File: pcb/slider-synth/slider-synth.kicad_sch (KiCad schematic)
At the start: 21 parts, among them J1 USB4105, J2 PJ-325C5-G, J3 Conn_01x02_Pin, SW1 SW_SPST, SW2 SW_SPST, U1 ESP32-S3-WROOM-2, U2 LM3940IMPX-3.3/NOPB

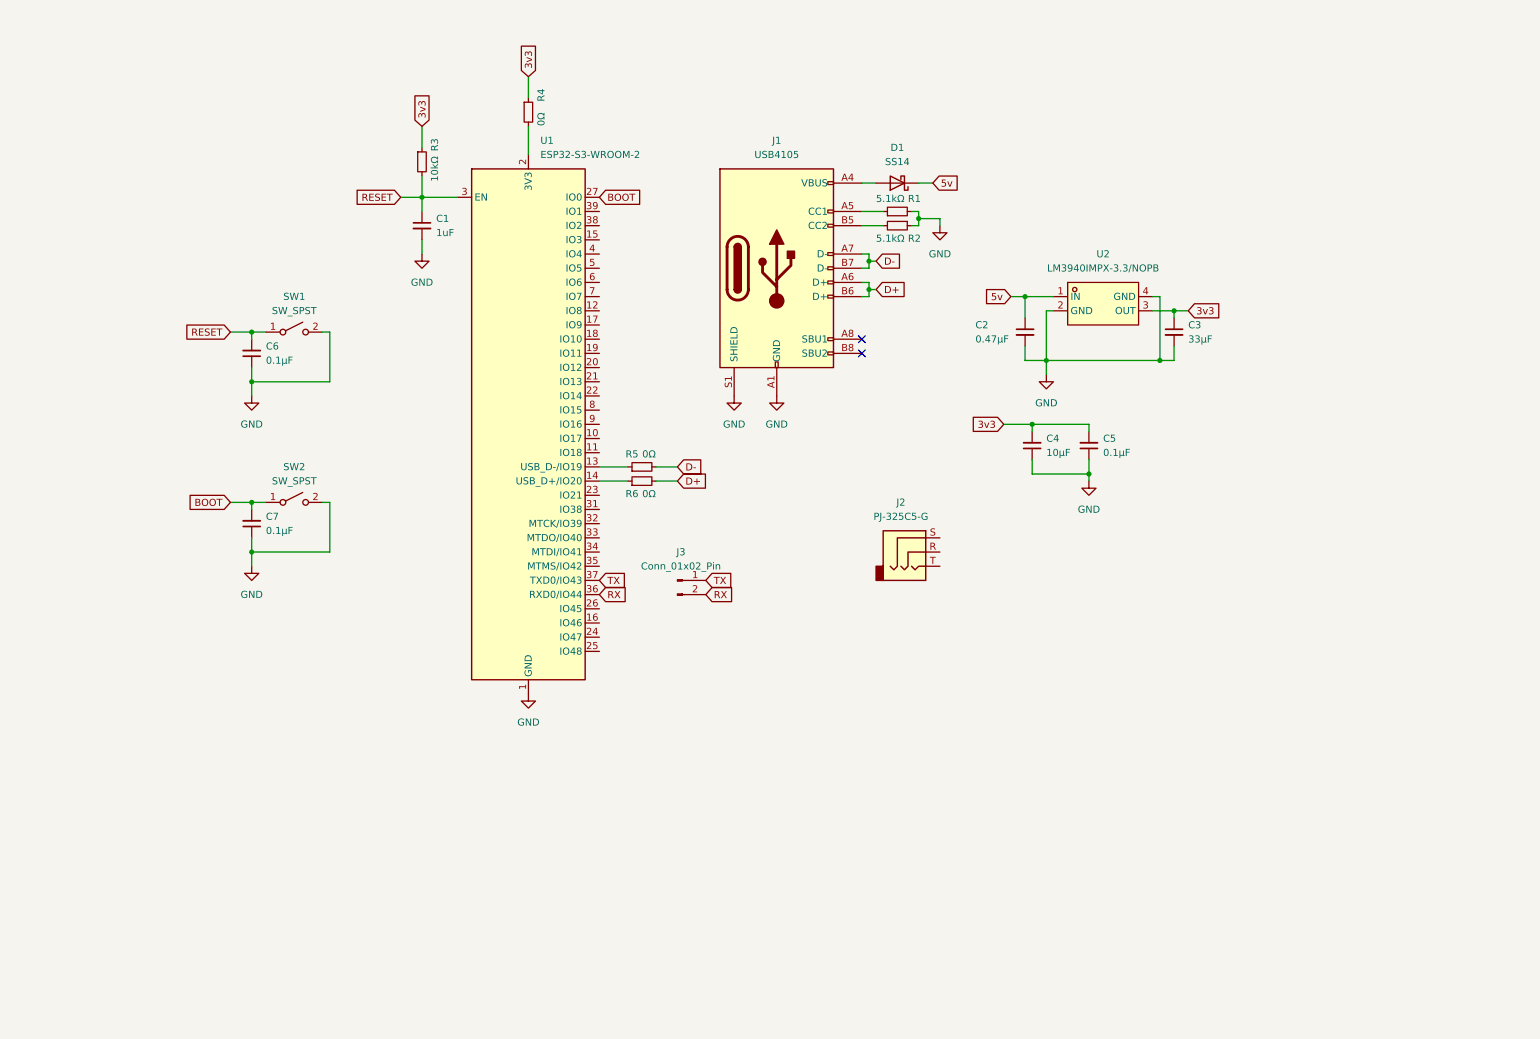
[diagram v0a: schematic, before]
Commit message: update schem
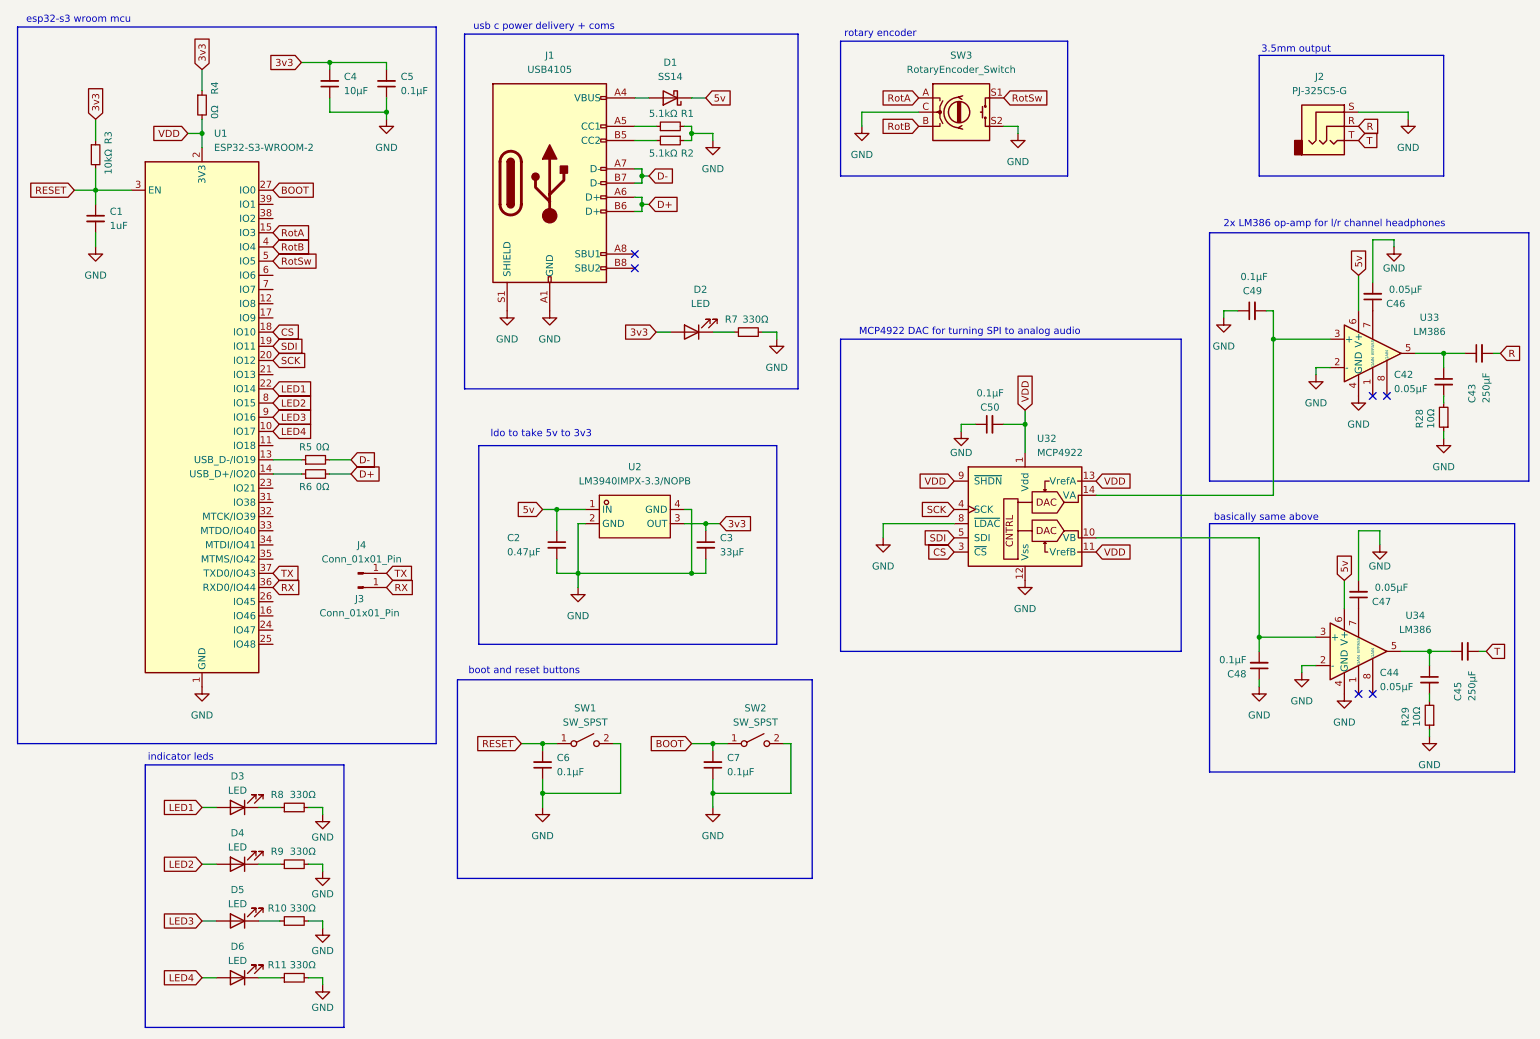
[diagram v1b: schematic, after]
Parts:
- removed J3: Conn_01x02_Pin, symbol Connector:Conn_01x02_Pin
- added C42, C44, C46, C47: 0.05μF, Capacitor_SMD:C_0805_2012Metric, symbol Device:C_Small
- added C43, C45: 250μF, Capacitor_SMD:C_0805_2012Metric, symbol Device:C_Small
- added C48, C49, C50: 0.1μF, Capacitor_SMD:C_0805_2012Metric, symbol Device:C_Small
- added D2, D3, D4, D5, D6: LED, LED_THT:LED_D5.0mm, symbol Device:LED
- added J3, J4: Conn_01x01_Pin, Connector_PinHeader_2.54mm:PinHeader_1x01_P2.54mm_Vertical, symbol Connector:Conn_01x01_Pin
- added R10, R11, R7, R8, R9: 330Ω, Resistor_SMD:R_0805_2012Metric, symbol Device:R_Small
- added R28, R29: 10Ω, Resistor_SMD:R_0805_2012Metric, symbol Device:R_Small
- added SW3: RotaryEncoder_Switch, Rotary_Encoder:RotaryEncoder_Alps_EC11E-Switch_Vertical_H20mm, symbol Device:RotaryEncoder_Switch
- added U32: MCP4922, Package_SO:SOIC-14_3.9x8.7mm_P1.27mm, symbol Analog_DAC:MCP4922
- added U33, U34: LM386, Package_SO:SOIC-8_3.9x4.9mm_P1.27mm, symbol Amplifier_Audio:LM386
- SW1, SW2: footprint (none) -> Button_Switch_THT:SW_PUSH_6mm
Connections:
- net 3v3: now also D2.2 (A)
- net 5v: now also U33.6 (V+), U34.6 (V+)
- net GND: now also J2.S, C46.2, C47.2, C48.1, C49.1, C50.1, R10.2, R11.2, R28.1, R29.1, R7.2, R8.2, R9.2, SW3.C, SW3.S2, U32.12 (Vss), U32.8 (~{LDAC}), U33.2 (-), U33.4 (GND), U34.2 (-), U34.4 (GND)
- net RX: now also J3.1 (Pin_1)
- net TX: now also J4.1 (Pin_1)
- net LED4: now reaches U1.10 (IO17)
- net LED4: now also D6.2 (A)
- net RotA: now reaches U1.15 (IO3)
- net RotA: now also SW3.A
- net CS: now reaches U1.18 (IO10)
- net CS: now also U32.3 (~{CS})
- net SDI: now reaches U1.19 (IO11)
- net SDI: now also U32.5 (SDI)
- net VDD: now reaches R4.2, U1.2 (3V3)
- net VDD: now also C50.2, U32.1 (Vdd), U32.11 (VrefB), U32.13 (VrefA), U32.9 (~{SHDN})
- net SCK: now reaches U1.20 (IO12)
- net SCK: now also U32.4 (SCK)
- net LED1: now reaches U1.22 (IO14)
- net LED1: now also D3.2 (A)
- net RotB: now reaches U1.4 (IO4)
- net RotB: now also SW3.B
- net RotSw: now reaches U1.5 (IO5)
- net RotSw: now also SW3.S1
- net LED2: now reaches U1.8 (IO15)
- net LED2: now also D4.2 (A)
- net LED3: now reaches U1.9 (IO16)
- net LED3: now also D5.2 (A)
- net R: now reaches J2.R
- net R: now also C43.2
- net T: now reaches J2.T
- net T: now also C45.2
- new net: C44.1, C45.1, U34.5
- new net: D3.1 (K), R8.1
- new net: C47.1, U34.7 (BYPASS)
- new net: C42.1, C43.1, U33.5
- new net: C42.2, R28.2
- new net: D5.1 (K), R10.1
- new net: C48.2, U32.10 (VB), U34.3 (+)
- new net: C49.2, U32.14 (VA), U33.3 (+)
- new net: C44.2, R29.2
- new net: D4.1 (K), R9.1
- new net: C46.1, U33.7 (BYPASS)
- new net: D6.1 (K), R11.1
- new net: D2.1 (K), R7.1
- no-connect marks 2 -> 6
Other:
- note added: "2x LM386 op-amp for l/r channel headphones"
- note added: "3.5mm output"
- note added: "MCP4922 DAC for turning SPI to analog audio"
- note added: "basically same above"
- note added: "boot and reset buttons"
- note added: "esp32-s3 wroom mcu"
- note added: "indicator leds"
- note added: "ldo to take 5v to 3v3"
- note added: "rotary encoder"
- note added: "usb c power delivery + coms"
- moved on the sheet: C1, C2, C3, C4, C5, C6, C7, D1, J1, J2, R1, R2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
